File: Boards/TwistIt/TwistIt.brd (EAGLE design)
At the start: 39.9 x 54.8 mm, 21 parts

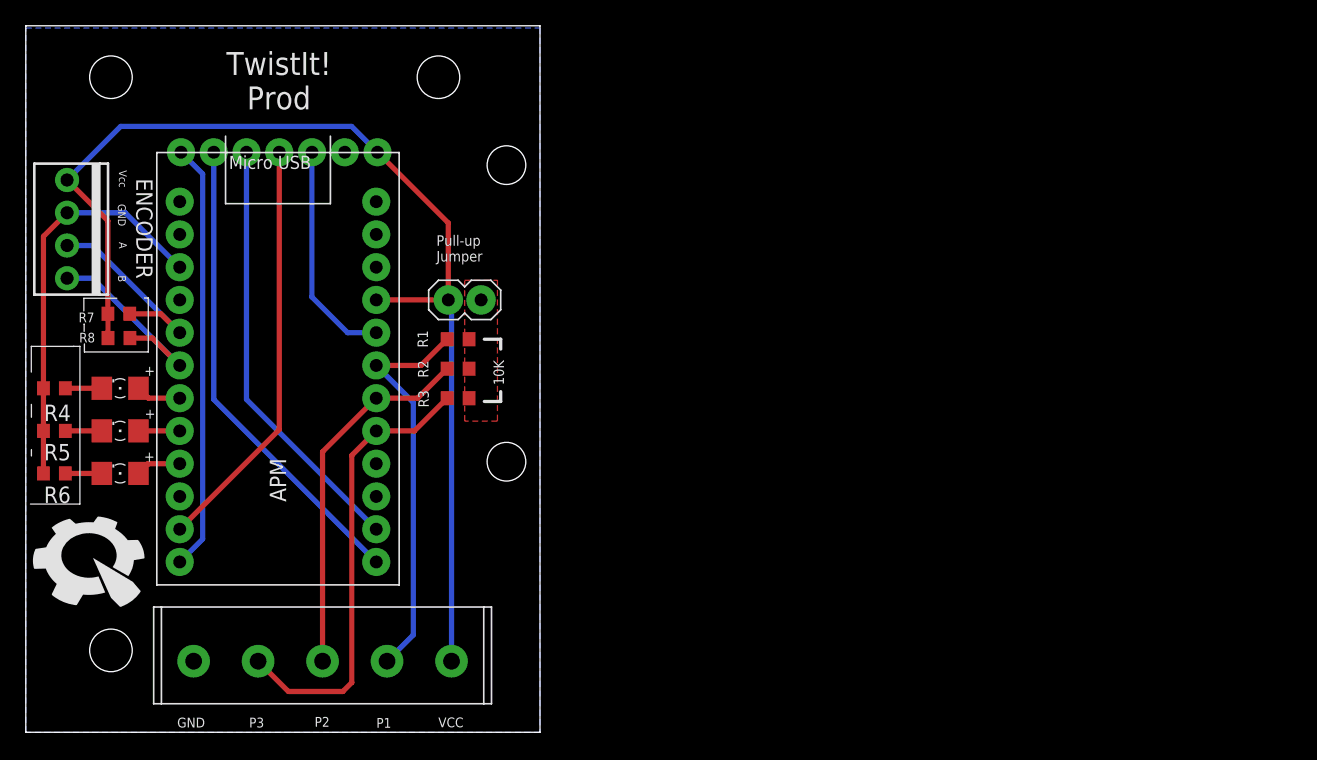
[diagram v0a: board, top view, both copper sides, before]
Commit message: cronCH
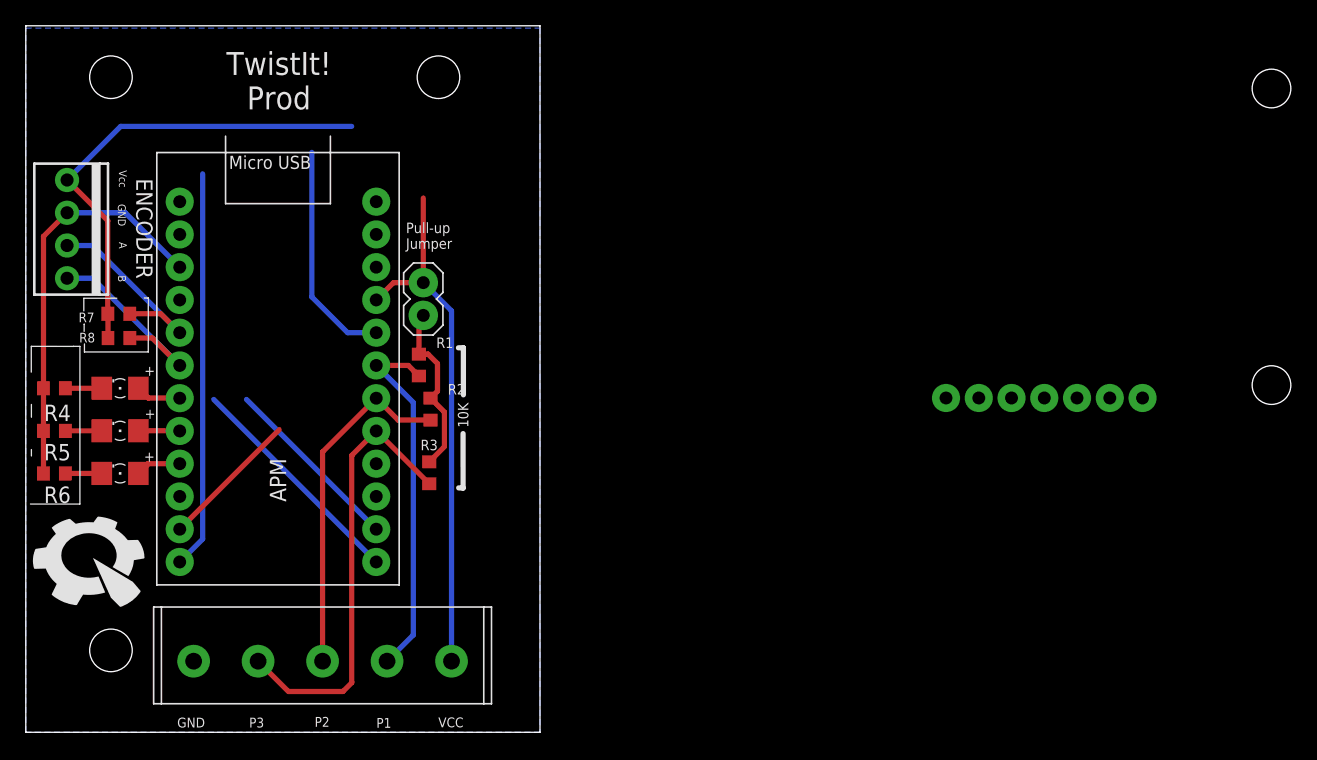
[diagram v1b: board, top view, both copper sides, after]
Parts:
- moved BR1 63.3 mm to (45.1, 24.4), flipped to the top, turned to 0 degrees
- moved R3 6.20 mm to (31.3, 20.1), turned to 90 degrees
- moved R2 3.80 mm to (31.4, 25.1), turned to 90 degrees
- moved R1 3.64 mm to (30.5, 28.5), turned to 90 degrees
- moved 5V_JUMPER 3.21 mm to (30.8, 33.6), turned to 270 degrees
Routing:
- net CS: track 32.4 -> 10.9 mm
- net INB: track 37.0 -> 17.8 mm
- net INA: track 33.4 -> 14.2 mm
- net 5V: track 0.00 -> 13.7 mm
- net VCC: track 87.6 -> 78.4 mm
- net P1: track 31.3 -> 28.6 mm
- net PWM: track 33.2 -> 30.8 mm
- net P2: track 28.6 -> 27.0 mm
- net P3: track 35.4 -> 34.6 mm
- removed copper zone on layer 1, net 5V
